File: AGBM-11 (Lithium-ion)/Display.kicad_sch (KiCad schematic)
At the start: 17 parts, among them P2 FFC CONNECTOR

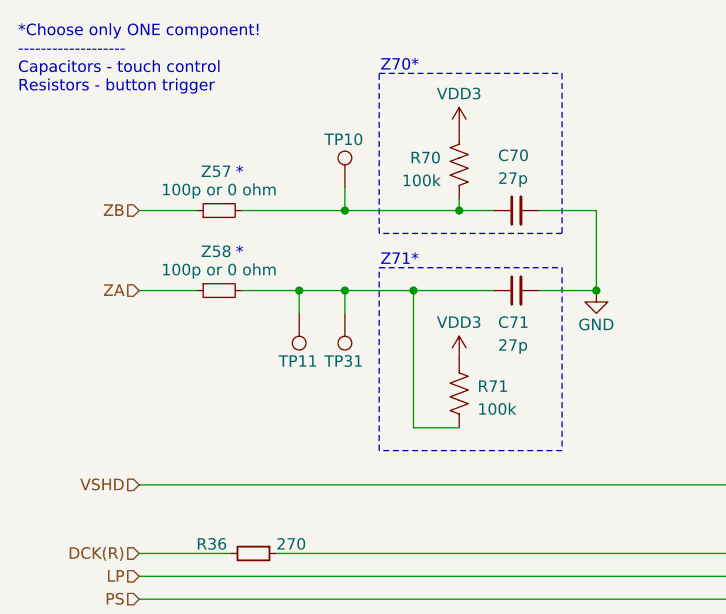
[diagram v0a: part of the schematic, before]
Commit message: Add files via upload
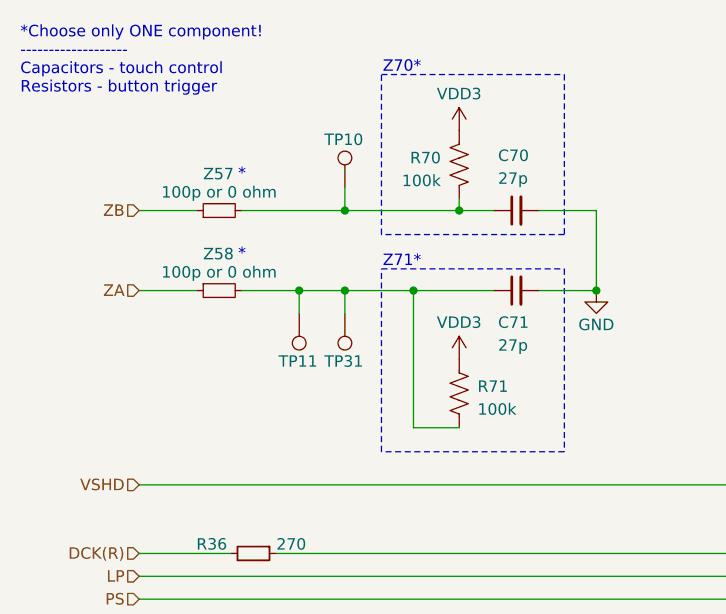
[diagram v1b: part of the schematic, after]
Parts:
- C11: Source https://www.digikey.com/short/2ppmm3vt -> (none)
- C13, C14: Source https://www.digikey.com/short/m958w3z3 -> (none)
- C70, C71: Source https://www.digikey.com/short/3dr3j004 -> (none)
- P2: Source https://www.digikey.com/short/13cnr9vq -> (none)
- R26: Source https://www.digikey.com/short/t0dpzzp1 -> (none)
- R36: Source https://www.digikey.com/short/85p4bp5h -> (none)
- R67, R70, R71: Source https://www.digikey.com/short/rpz9t4md -> (none)
- TP11: footprint Bucketmouse:TestPoint_Pad_D1.25mm_VIA -> Bucketmouse:TestPoint_Pad_D1.0mm_VIA
- VR1: footprint OpenTendo-AGB:VR1 -> Bucketmouse:3313J-2; Source https://www.digikey.com/short/p8zptq5h -> (none)
- Z57, Z58: Source https://www.digikey.com/short/h34j0h9q -> (none)
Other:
- company: https://github.com/MouseBiteLabs/Game-Boy-Enhance -> https://github.com/MouseBiteLabs/Game-Boy-Enhance/
- title: Game Boy Enhance (AGBM-01) -> Game Boy Enhance (AGBM-11)
